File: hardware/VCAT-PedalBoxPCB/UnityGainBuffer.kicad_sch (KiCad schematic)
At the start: 8 parts, among them U3 TLV9301xDCK

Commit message: updated mx150 pin order :( works now
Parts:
- C1, C3, R4: P/N pickle -> (none)
- R11, R2: P/N ERA-3ARB822V -> (none)

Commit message: updated BOM
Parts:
- C1: P/N (none) -> MSASH168SB5103KTNA01
- C3: P/N (none) -> MLASH168SB7104KTNA01
- R11: P/N (none) -> CRCW0402100RFKEDHP
- R2: P/N (none) -> CRCW060310K0FKEI
- R4: P/N (none) -> CRCW060322K0FKEAHP
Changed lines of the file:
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@@
 			)
 		)
-		(property "Description" "Unpolarized capacitor"
+		(property "Description" "Pedals BrakePot C2 cap"
 			(at 151.765 100.965 0)
 			(effects
@@
 			)
 		)
-		(property "P/N" ""
+		(property "P/N" "MLASH168SB7104KTNA01"
 			(at 151.765 100.965 0)
 			(effects
@@
 			)
 		)
-		(property "Description" "Unpolarized capacitor"
+		(property "Description" "Pedal BrakePot C6 cap"
 			(at 178.435 114.935 0)
 			(effects
@@
 			)
 		)
-		(property "P/N" ""
+		(property "P/N" "MSASH168SB5103KTNA01"
 			(at 178.435 114.935 0)
 			(effects
@@
 			)
 		)
-		(property "Description" "40-V, 1-MHz, RRO Operational Amplifiers for Cost-Sensitive Systems, SC-70"
+		(property "Description" "TLV9301IDCKR"
 			(at 147.955 111.125 0)
 			(effects
@@
 			)
 		)
-		(property "Description" "Resistor, US symbol"
+		(property "Description" "Pedals 22k ohms"
 			(at 127.635 113.665 0)
 			(effects
@@
 			)
 		)
-		(property "P/N" ""
+		(property "P/N" "CRCW060322K0FKEAHP"
 			(at 127.635 113.665 0)
 			(effects
@@
 			)
 		)
-		(property "Description" "Resistor, US symbol"
+		(property "Description" "Pedals 10K Ohms"
 			(at 122.555 108.585 0)
 			(effects
@@
 			)
 		)
-		(property "P/N" ""
+		(property "P/N" "CRCW060310K0FKEI "
 			(at 122.555 108.585 0)
 			(effects
@@
 			)
 		)
-		(property "Description" "Resistor, US symbol"
+		(property "Description" "Pedals 100 ohms"
 			(at 171.45 111.125 0)
 			(effects
@@
 			)
 		)
-		(property "P/N" ""
+		(property "P/N" "CRCW0402100RFKEDHP"
 			(at 171.45 111.125 0)
 			(effects

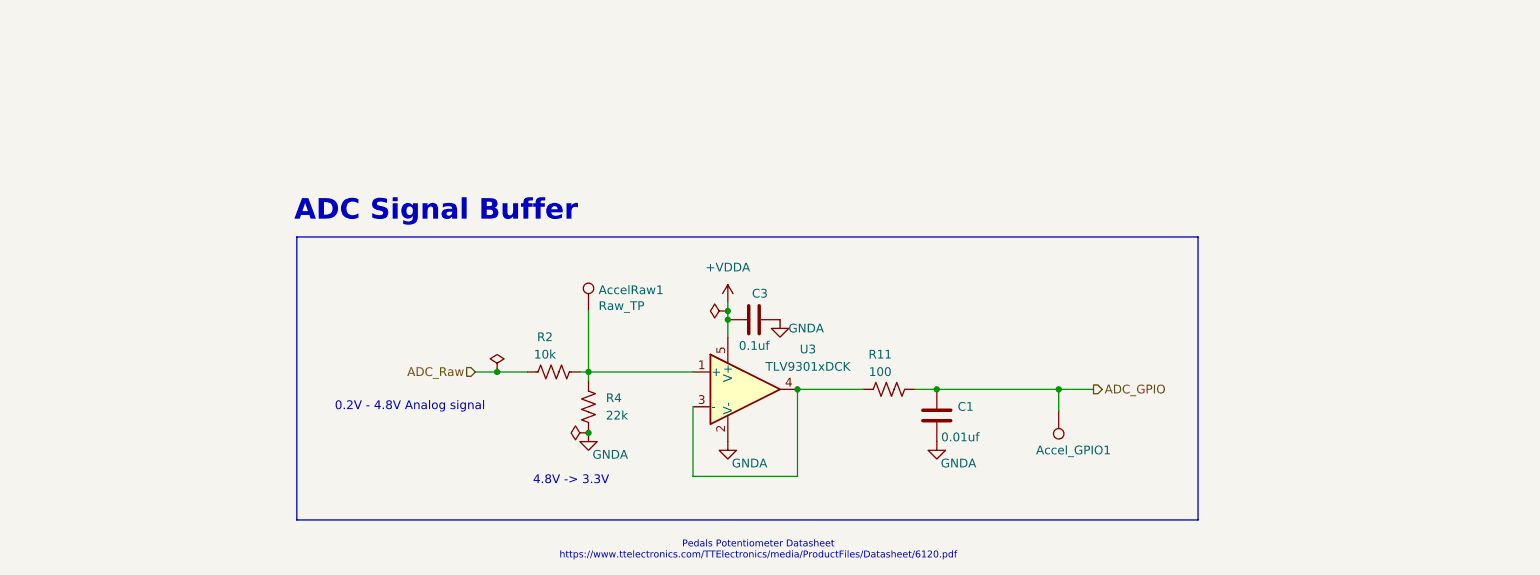
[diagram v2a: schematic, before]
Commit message: bruh
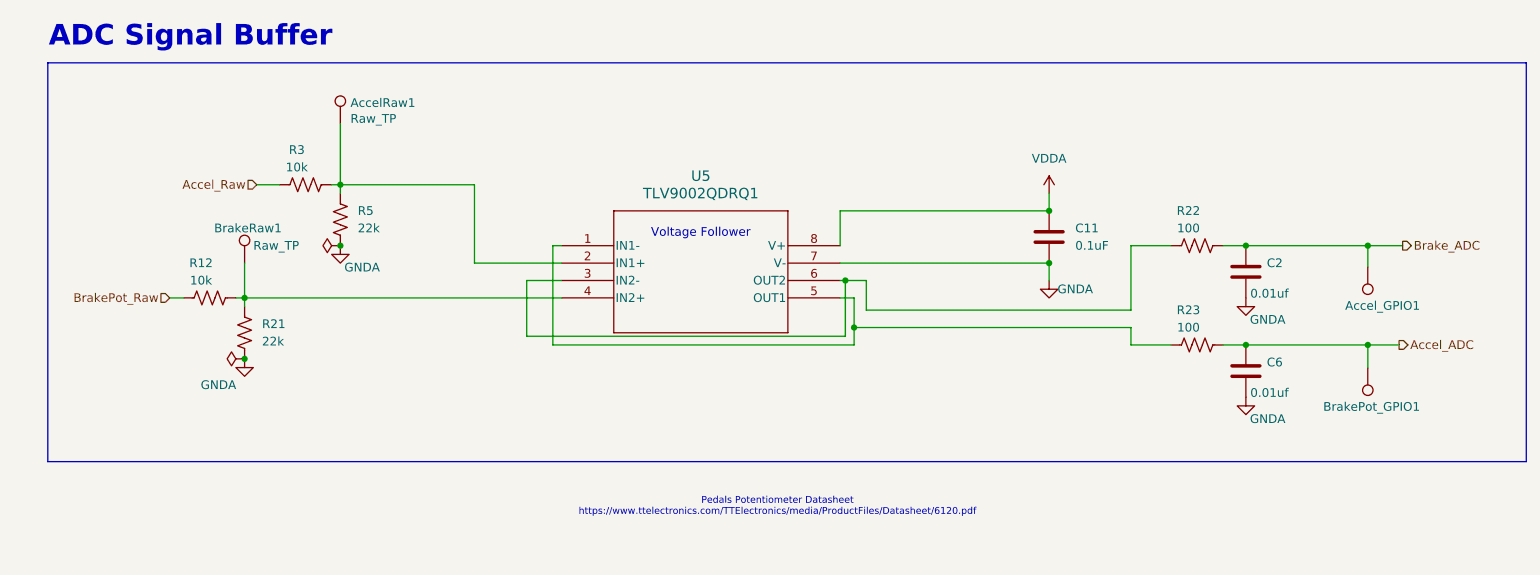
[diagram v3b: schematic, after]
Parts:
- removed C1: 0.01uf, Capacitor_SMD:C_0603_1608Metric_Pad1.08x0.95mm_HandSolder, symbol Device:C
- removed C3: 0.1uf, Capacitor_SMD:C_0603_1608Metric_Pad1.08x0.95mm_HandSolder, symbol Device:C
- removed R11: 100, Resistor_SMD:R_0603_1608Metric_Pad0.98x0.95mm_HandSolder, symbol Device:R_US
- removed R2: 10k, Resistor_SMD:R_0603_1608Metric_Pad0.98x0.95mm_HandSolder, symbol Device:R_US
- removed R4: 22k, Resistor_SMD:R_0603_1608Metric_Pad0.98x0.95mm_HandSolder, symbol Device:R_US
- removed U3: TLV9301xDCK, Package_TO_SOT_SMD:SOT-353_SC-70-5, symbol Amplifier_Operational:TLV9301xDCK
- added BrakePot_GPIO1: Accel, TestPoint:TestPoint_THTPad_1.5x1.5mm_Drill0.7mm, symbol Connector:TestPoint
- added BrakeRaw1: Raw_TP, TestPoint:TestPoint_THTPad_1.5x1.5mm_Drill0.7mm, symbol Connector:TestPoint
- added C11: 0.1uF, Capacitor_SMD:C_0603_1608Metric_Pad1.08x0.95mm_HandSolder, symbol Device:C
- added C2, C6: 0.01uf, Capacitor_SMD:C_0603_1608Metric_Pad1.08x0.95mm_HandSolder, symbol Device:C
- added R12, R3: 10k, Resistor_SMD:R_0603_1608Metric_Pad0.98x0.95mm_HandSolder, symbol Device:R_US
- added R21, R5: 22k, Resistor_SMD:R_0603_1608Metric_Pad0.98x0.95mm_HandSolder, symbol Device:R_US
- added R22, R23: 100, Resistor_SMD:R_0603_1608Metric_Pad0.98x0.95mm_HandSolder, symbol Device:R_US
- added U5: TLV9002QDRQ1, TLV9002QDRQ1:SOIC8_D_TEX, symbol TLV9002QDRQ1:TLV9002QDRQ1
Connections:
- net GNDA: now also C11.2, C2.1, C6.1, R21.2, R5.2, U5.7 (V-)
- net at AccelRaw1.1: now also R3.1, R5.1, U5.2 (IN1+)
- net ADC_GPIO renamed Brake_ADC
- net Brake_ADC: now also C2.2, R22.1
- new net: R23.2, U5.1 (IN1-), U5.5 (OUT1)
- new net: BrakeRaw1.1, R12.1, R21.1, U5.4 (IN2+)
- new net: R22.2, U5.3 (IN2-), U5.6 (OUT2)
- new net Accel_ADC: BrakePot_GPIO1.1, C6.2, R23.1
- new net Accel_Raw: R3.2
- new net BrakePot_Raw: R12.2
- new net VDDA: C11.1, U5.8 (V+)
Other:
- note added: "Voltage Follower"
- note removed: "0.2V - 4.8V Analog signal"
- note removed: "4.8V -> 3.3V"
- moved on the sheet: AccelRaw1
